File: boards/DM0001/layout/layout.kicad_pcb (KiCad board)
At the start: 6 copper layers, 24.9 x 51.5 mm, 147 parts, among them IC1 TCAN330DCNT, IC2 LDFPVR, IC3 LDFPVR, IC4 L6387ED, IC5 L6387ED, IC6 L6387ED, IC7 STM32G431C8T6, J1 BM05B-SRSS-TB, J2 BM05B-SRSS-TB, J3 SM05B-SRSS-TB, J4 ?, Q1 STL180N6F7, Q2 STL180N6F7, Q3 STL180N6F7, Q4 STL180N6F7, Q5 STL180N6F7, Q6 STL180N6F7, Y1 CSTNE8M00GH5C000R0

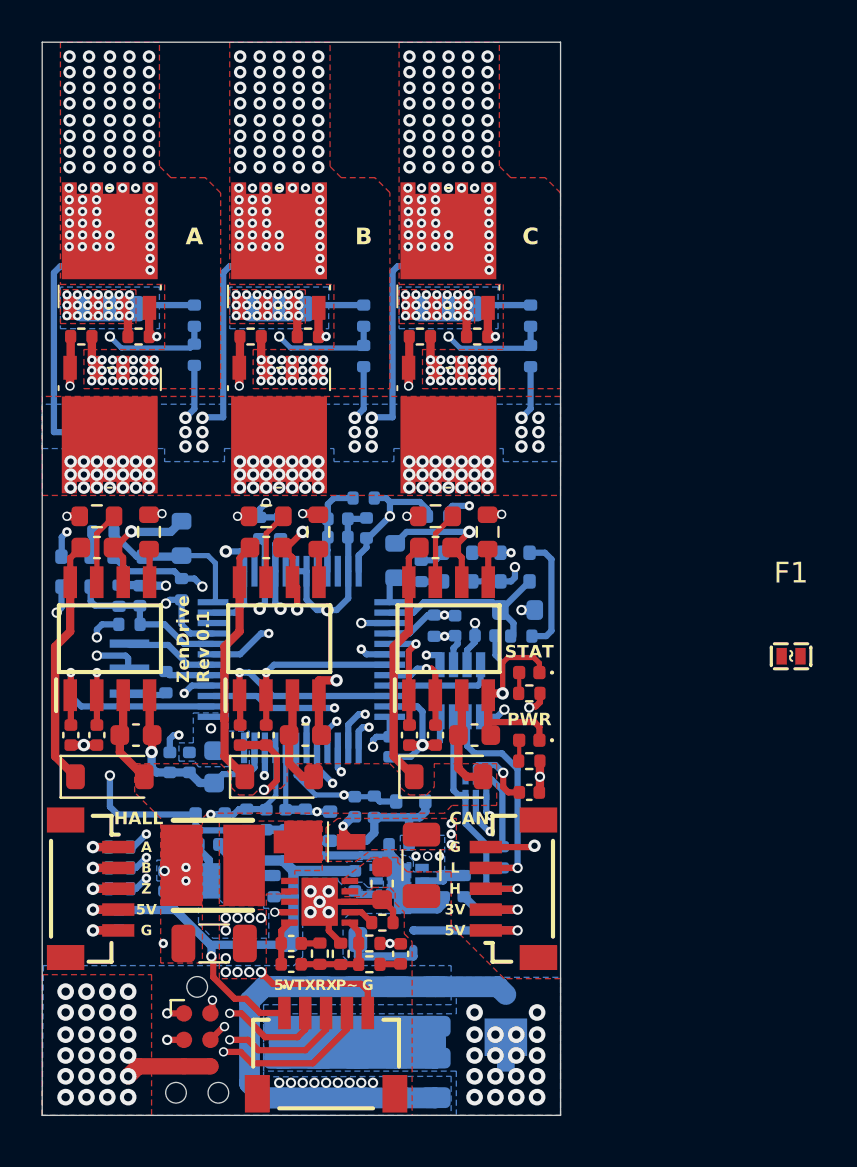
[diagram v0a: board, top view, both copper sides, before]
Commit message: update stdlib
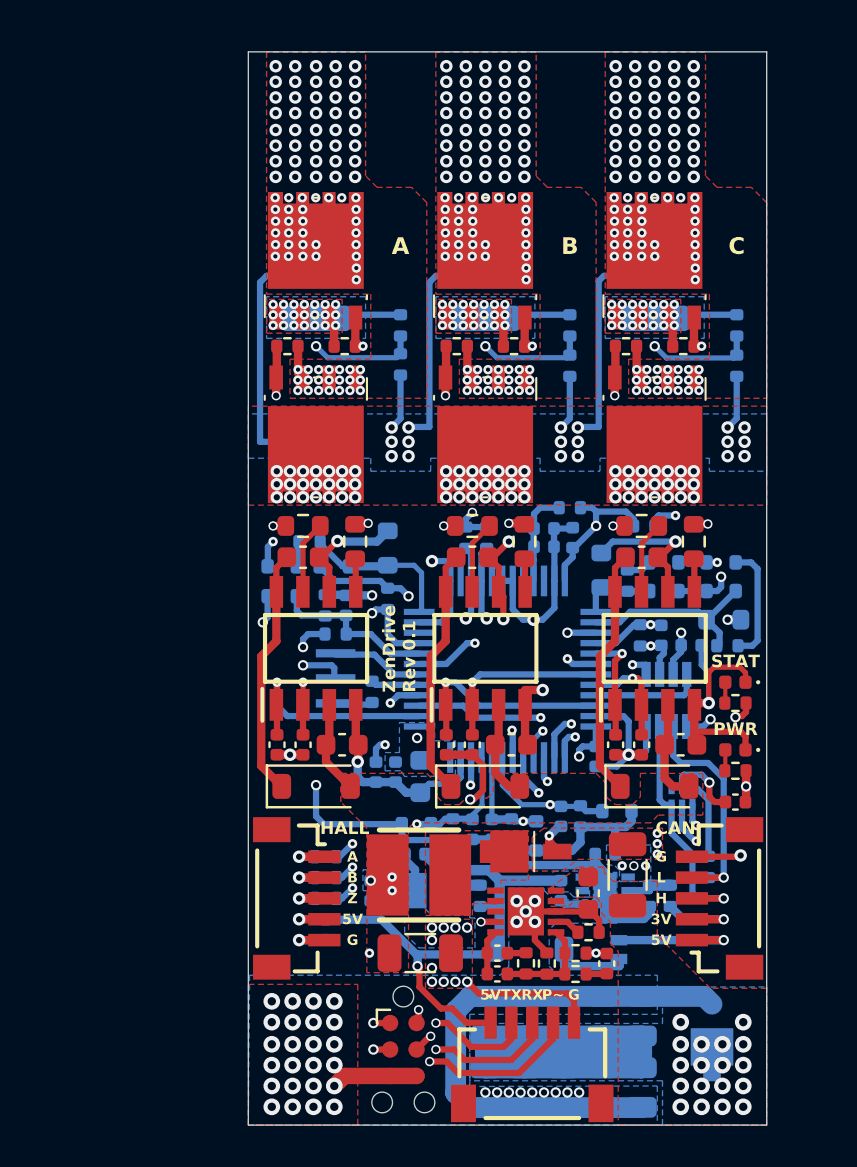
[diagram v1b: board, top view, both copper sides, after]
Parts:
- F1: moved to B.Cu
- moved F1 16.3 mm to (82.4, 120.4), turned to 90 degrees
- moved C1 9.90 mm to (82.8, 116.9)
- moved C10 9.90 mm to (85.9, 105.8)
- moved C11 9.90 mm to (79.6, 114.0)
- moved C12 9.90 mm to (76.3, 114.7)
- moved C13 9.90 mm to (75.4, 114.7)
- moved C14 9.90 mm to (68.3, 119.5)
- moved C15 9.90 mm to (79.6, 117.6)
- moved C16 9.90 mm to (81.7, 115.9)
- moved C2 9.90 mm to (80.9, 117.7)
- moved C24 9.90 mm to (76.0, 88.1)
- moved C25 9.90 mm to (75.4, 101.6)
- moved C26 9.90 mm to (75.4, 110.6)
- moved C27 9.90 mm to (74.1, 110.6)
- moved C28 9.90 mm to (77.2, 110.6)
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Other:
- board text added: "0.0152 mm"
- board text added: "0.025"
- board text added: "0.0900 mm / 0.0900 mm"
- board text added: "0.0994 mm"
- board text added: "0.1164 mm"
- board text added: "0.1500 mm"
- board text added: "0.55 mm"
- board text added: "2116"
- board text added: "3313"
- board text added: "4.1"
- board text added: "4.16"
- board text added: "4.6"
- board text added: "Black"
- board text added: "ENIG"
- board text added: "FR4-Core"
- board text added: "White"
- board text removed: "0.02"
- board text removed: "0.1 mm"
- board text removed: "0.1600 mm / 0.2000 mm"
- board text removed: "0.2000 mm"
- board text removed: "0.535 mm"
- board text removed: "4.5"
- board text removed: "FR4"
- board text removed: "None"
